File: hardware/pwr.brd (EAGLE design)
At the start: 38 x 28 mm, 21 parts, among them IC2 LM2675M-ADJ, Q2 IRFR5305, T1 BC846, T2 BC846, X3 MKDSN1,5/4-5,08

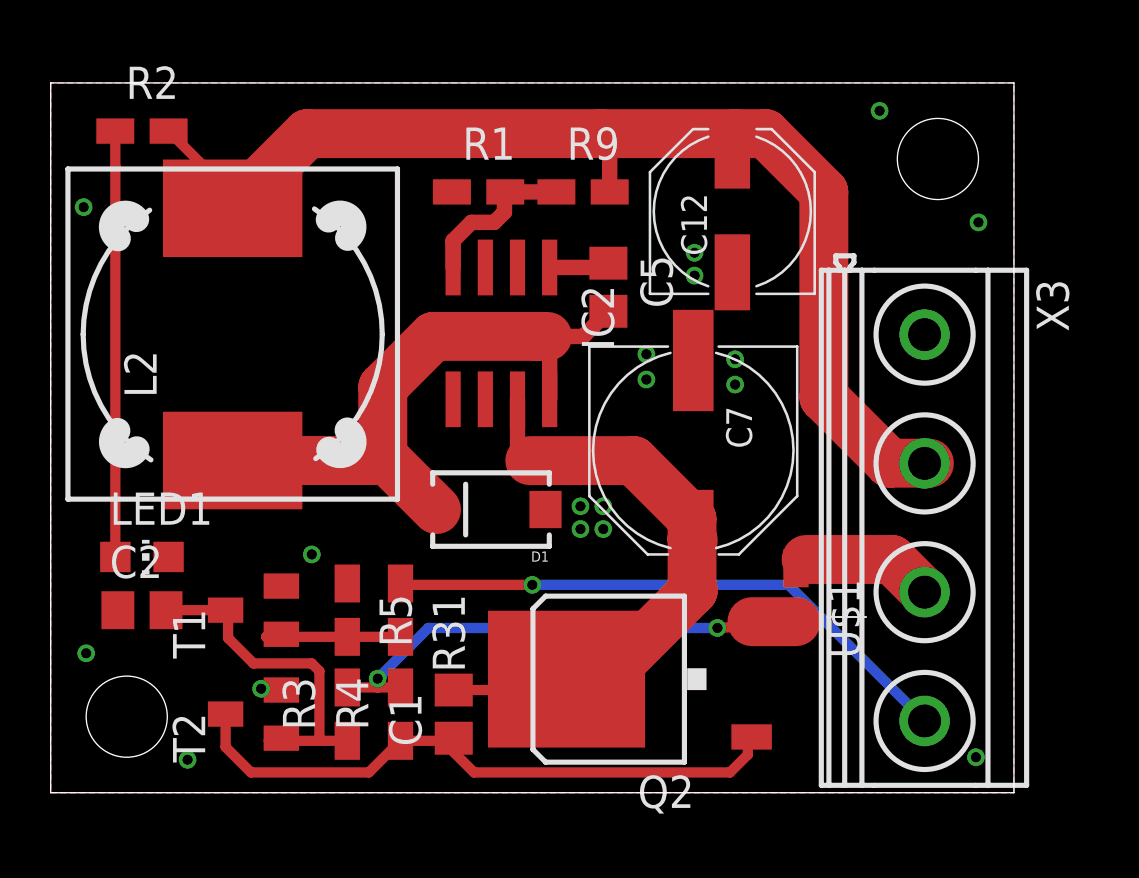
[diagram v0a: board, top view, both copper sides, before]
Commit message: board ready
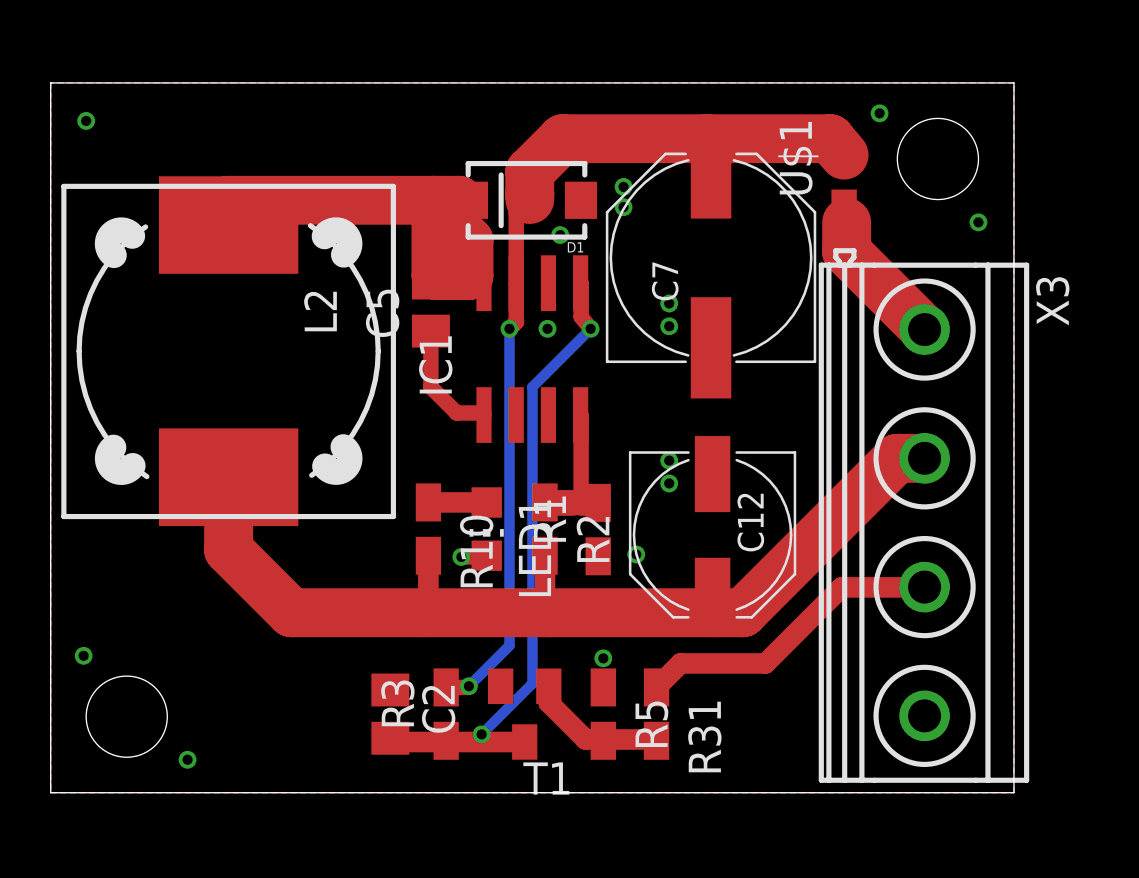
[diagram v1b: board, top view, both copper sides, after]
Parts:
- removed C1: 10nF, rcl:C0805
- removed IC2: LM2675M-ADJ, Simplex-ICs:SO-08
- removed Q2: IRFR5305, transistor-power:D-PAK_TO252AA
- removed R4: 220k, rcl:R0805W
- removed R9: 4.75k 1%, rcl:R0805W
- removed T2: BC846, transistor:SOT23
- added IC1: (no value), Simplex-ICs:SO-08
- added R10: 200k, rcl:R0805W
- R2: value 200k -> 4k
- moved R2 22.3 mm to (19.5, 10.4), turned to 270 degrees
- moved U$1 16.4 mm to (31.3, 24.1), turned to 90 degrees
- moved R1 14.1 mm to (21.6, 10.4), turned to 90 degrees
- moved LED1 13.6 mm to (17.2, 10.4), turned to 180 degrees
- moved C12 12.8 mm to (26.1, 10.2), turned to 270 degrees
- moved D1 12.3 mm to (18.8, 23.4)
- moved T1 11.5 mm to (18.7, 3.10), turned to 180 degrees
- moved R5 10.9 mm to (21.8, 3.10)
- moved R31 10.9 mm to (23.9, 3.10)
- moved C2 10.6 mm to (13.4, 3.10), turned to 270 degrees
- moved C7 7.63 mm to (26.1, 21.1), turned to 90 degrees
- moved C5 7.04 mm to (15.0, 19.2), turned to 90 degrees
- moved R3 3.90 mm to (15.6, 3.10)
- moved L2 0.68 mm to (7.02, 17.4), turned to 270 degrees
- moved X3 0.20 mm to (34.5, 10.6)
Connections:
- removed net N$16: C1.1, Q2.1, R4.1, T2.3
- removed net N$5: Q2.3, R3.2, R4.2, U$1.2
- net CE: now also X3.3; no longer X3.4
- net GND: now also IC1.2, IC1.3, IC1.6, X3.4; no longer IC2.6, T2.2, X3.1
- net N$1: now also R10.1; no longer R2.1
- net N$10: now also IC1.1; no longer IC2.1
- net N$2: now also IC1.5; no longer T2.1
- net N$4: now also IC1.4, R2.1; no longer IC2.4, R9.1
- net N$49: now also IC1.7, R3.2, U$1.2; no longer C1.2, IC2.7, Q2.4
- net N$9: now also IC1.8; no longer IC2.8
- net V_IN: now also X3.1; no longer X3.3
- net V_OUT: now also R10.2; no longer R9.2
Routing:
- net N$16: track 25.2 -> 0.00 mm
- net N$5: track 19.9 -> 0.00 mm, vias 2 -> 0
- net N$1: track 16.8 -> 2.30 mm
- net N$2: track 14.0 -> 26.6 mm, vias 0 -> 2
- net CE: track 22.9 -> 12.2 mm, vias 1 -> 0
- net N$49: track 28.1 -> 37.6 mm, vias 0 -> 2
- net V_OUT: track 46.9 -> 39.5 mm
- net N$9: track 24.8 -> 19.0 mm
- net N$10: track 2.39 -> 4.76 mm
- net N$4: track 6.37 -> 5.58 mm
- net GND: track 0.82 -> 1.02 mm, vias 18 -> 16
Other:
- board text added: "R1"
- board text added: "R2"
- board text added: "V_IN = 6.5 - 40V V_OUT = 1.21(1+R2/R1)"
- board text added: "V_IN V_OUT CE GND"
